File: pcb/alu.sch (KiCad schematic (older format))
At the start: 19 parts

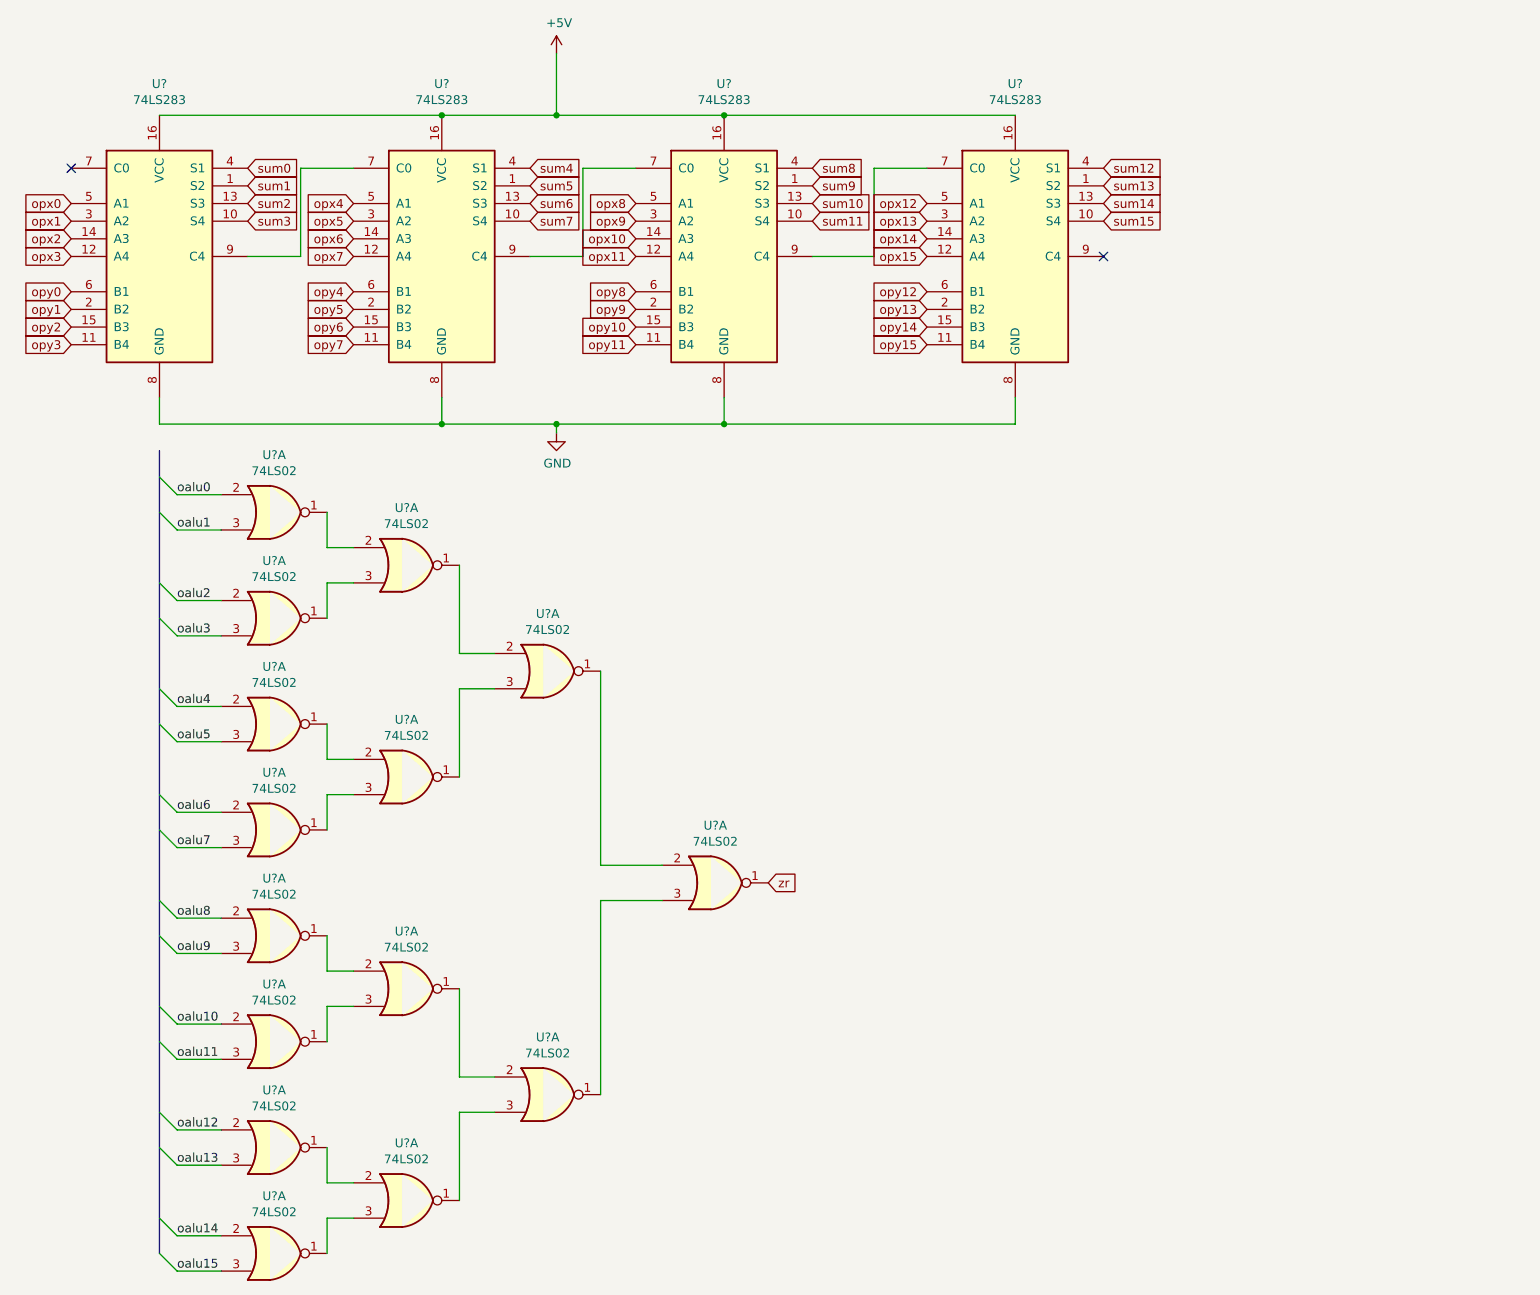
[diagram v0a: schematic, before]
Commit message: flash mem
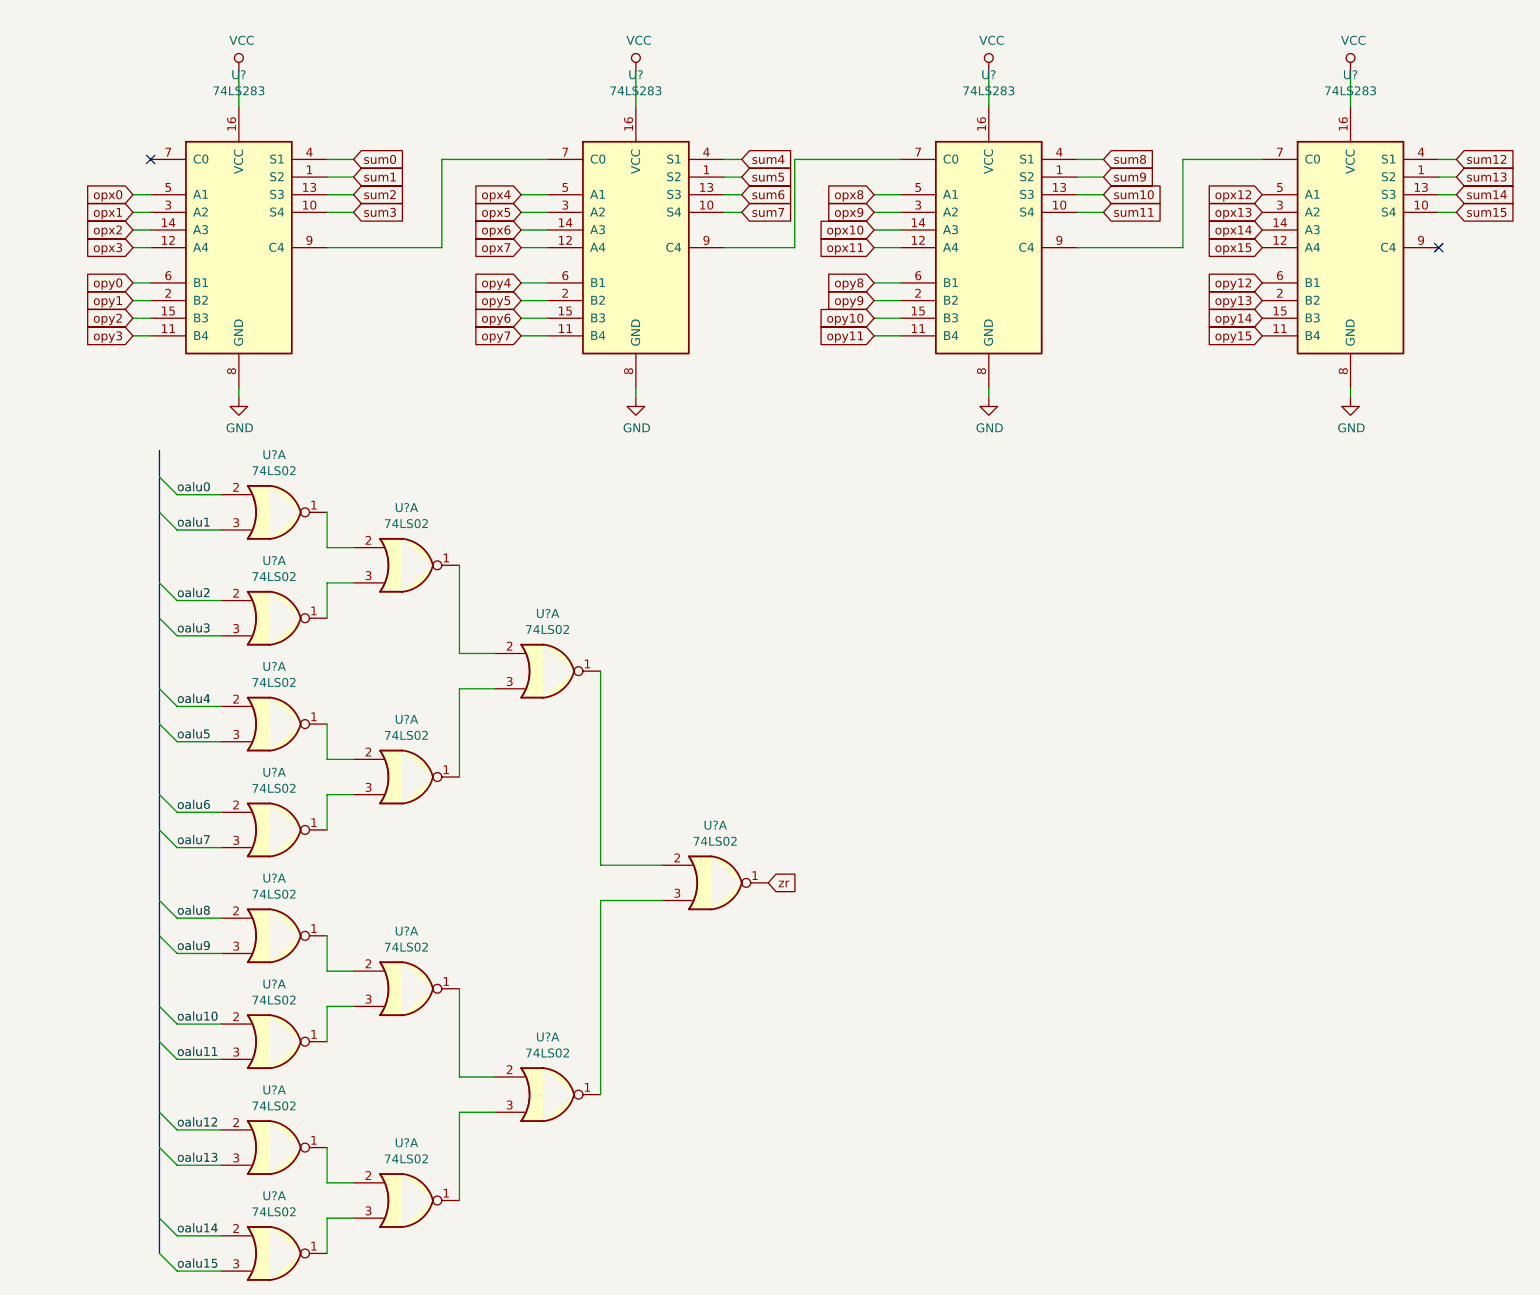
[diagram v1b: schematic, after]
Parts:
- removed U? (x4): 74LS283, Package_SO:SOIC-16_3.9x9.9mm_P1.27mm, symbol 74xx:74LS283
- added U? (x4): 74LS283, Package_SO:SOIC-16_3.9x9.9mm_P1.27mm, symbol 74xx:74LS283
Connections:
- net GND: now also U?.8 (GND), U?.8 (GND), U?.8 (GND), U?.8 (GND)
- net opx0: now also U?.5 (A1)
- net opx1: now also U?.3 (A2)
- net opx10: now also U?.14 (A3)
- net opx11: now also U?.12 (A4)
- net opx12: now also U?.5 (A1)
- net opx13: now also U?.3 (A2)
- net opx14: now also U?.14 (A3)
- net opx15: now also U?.12 (A4)
- net opx2: now also U?.14 (A3)
- net opx3: now also U?.12 (A4)
- net opx4: now also U?.5 (A1)
- net opx5: now also U?.3 (A2)
- net opx6: now also U?.14 (A3)
- net opx7: now also U?.12 (A4)
- net opx8: now also U?.5 (A1)
- net opx9: now also U?.3 (A2)
- net opy0: now also U?.6 (B1)
- net opy1: now also U?.2 (B2)
- net opy10: now also U?.15 (B3)
- net opy11: now also U?.11 (B4)
- net opy12: now also U?.6 (B1)
- net opy13: now also U?.2 (B2)
- net opy14: now also U?.15 (B3)
- net opy15: now also U?.11 (B4)
- net opy2: now also U?.15 (B3)
- net opy3: now also U?.11 (B4)
- net opy4: now also U?.6 (B1)
- net opy5: now also U?.2 (B2)
- net opy6: now also U?.15 (B3)
- net opy7: now also U?.11 (B4)
- net opy8: now also U?.6 (B1)
- net opy9: now also U?.2 (B2)
- net sum0: now also U?.4 (S1)
- net sum1: now also U?.1 (S2)
- net sum10: now also U?.13 (S3)
- net sum11: now also U?.10 (S4)
- net sum12: now also U?.4 (S1)
- net sum13: now also U?.1 (S2)
- net sum14: now also U?.13 (S3)
- net sum15: now also U?.10 (S4)
- net sum2: now also U?.13 (S3)
- net sum3: now also U?.10 (S4)
- net sum4: now also U?.4 (S1)
- net sum5: now also U?.1 (S2)
- net sum6: now also U?.13 (S3)
- net sum7: now also U?.10 (S4)
- net sum8: now also U?.4 (S1)
- net sum9: now also U?.1 (S2)
- new net: U?.7 (C0), U?.9 (C4) (x3)
- new net VCC: U?.16 (VCC), U?.16 (VCC), U?.16 (VCC), U?.16 (VCC)
